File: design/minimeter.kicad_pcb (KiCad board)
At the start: 2 copper layers, 44.4 x 26.7 mm, 14 parts, among them J1 Conn_01x02_Pin, J2 I2C, SW1 SW_Push_Dual, SW2 SW_Push_Dual

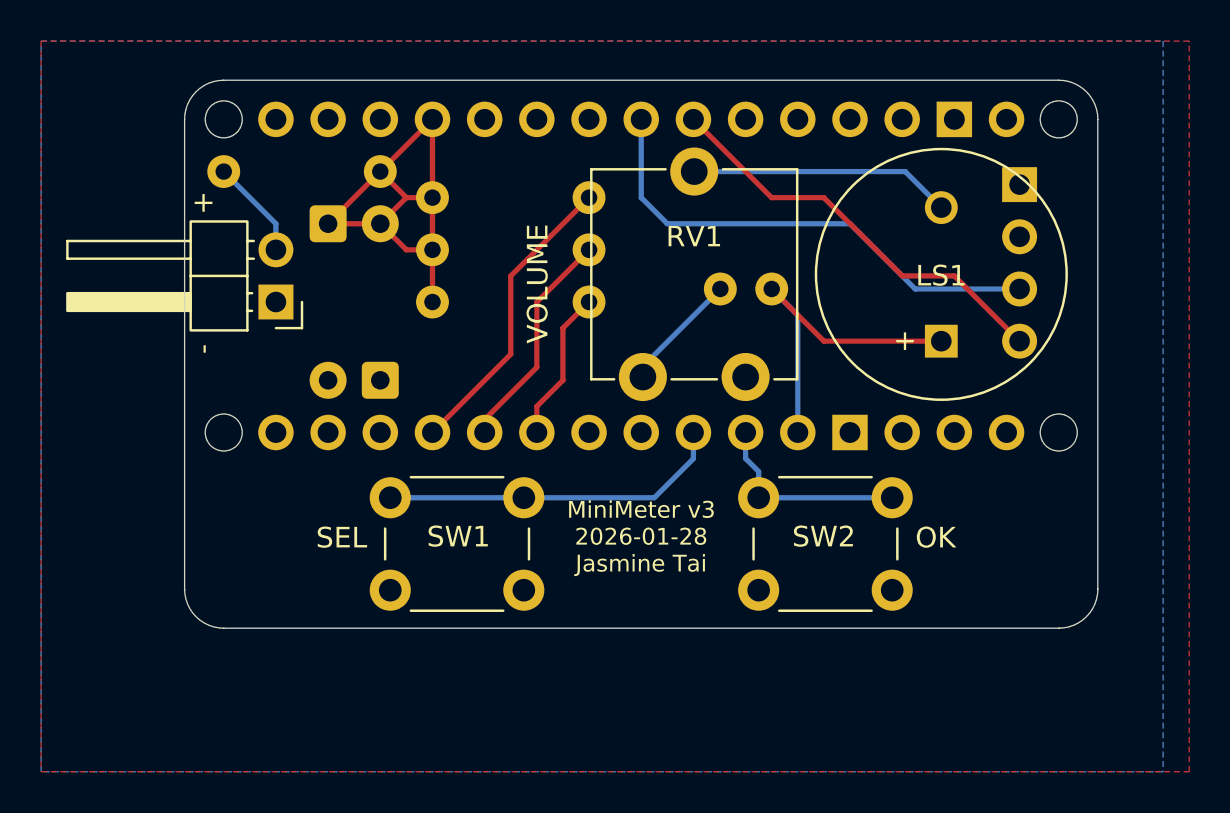
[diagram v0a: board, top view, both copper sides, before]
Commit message: Update design to v4
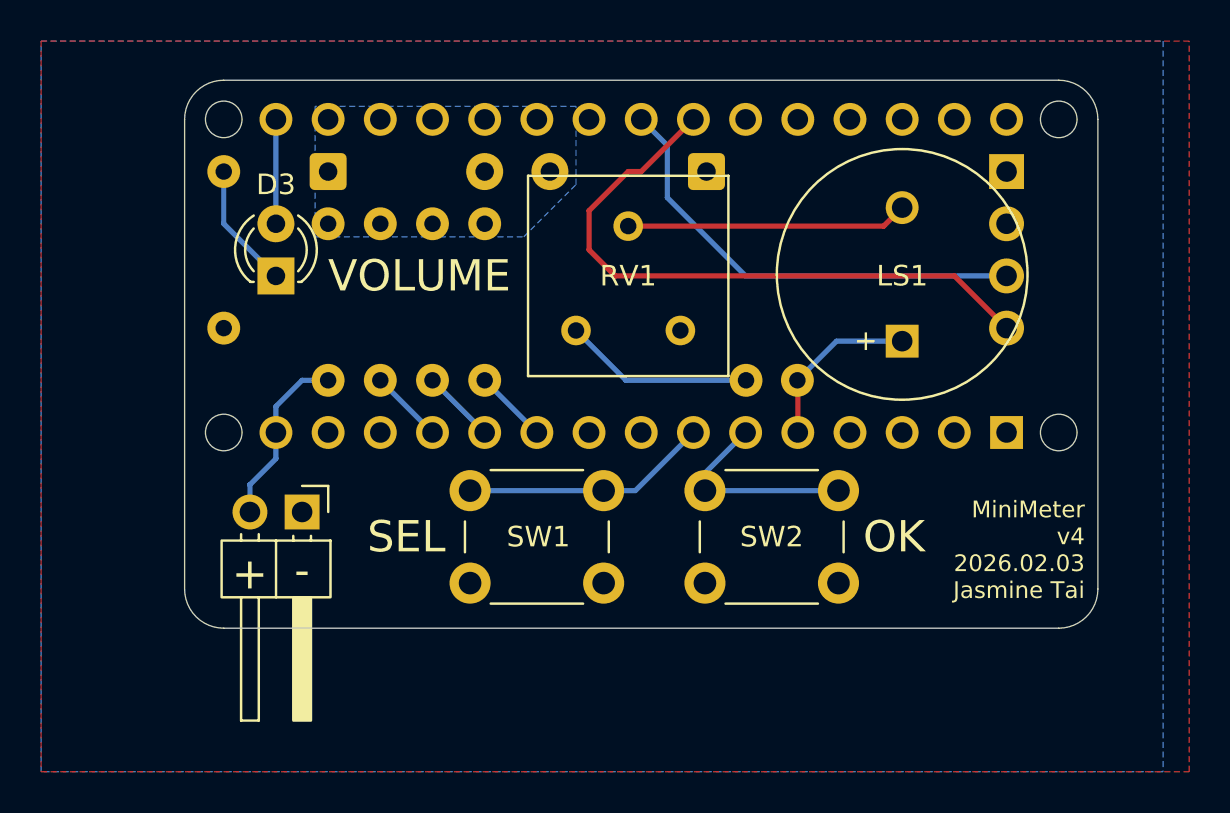
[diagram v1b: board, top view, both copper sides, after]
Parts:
- added D3: LED_Filled, LED_THT:LED_D3.0mm, F.Cu at (49.5, 57.1)
- added R5: 820, Resistor_THT:R_Axial_DIN0207_L6.3mm_D2.5mm_P7.62mm_Horizontal, B.Cu at (47.0, 59.7)
- A1: footprint arduino-library:Arduino_Nano_Socket -> Module:Arduino_Nano_WithMountingHoles
- RV1: footprint Potentiometer_THT:Potentiometer_ACP_CA9-V10_Vertical -> Potentiometer_THT:Potentiometer_Bourns_3386F_Vertical
- moved A1 40.1 mm to (85.1, 64.8)
- moved D1 18.8 mm to (70.5, 52.1), turned to 180 degrees
- moved R1 11.4 mm to (52.1, 62.2), turned to 90 degrees
- moved J1 10.3 mm to (50.8, 68.6), turned to -90 degrees
- moved C1 4.62 mm to (74.9, 62.2)
- moved R4 4.58 mm to (59.7, 54.6), turned to -90 degrees
- moved SW1 3.90 mm to (59.0, 67.6)
- moved RV1 3.90 mm to (69.2, 59.8)
- moved R2 2.84 mm to (54.6, 54.6), turned to -90 degrees
- moved SW2 2.64 mm to (70.4, 67.6)
- moved D2 2.54 mm to (52.1, 52.1), turned to 0 degrees
- moved LS1 1.91 mm to (80.0, 60.3)
- moved R3 1.27 mm to (57.1, 54.6), turned to -90 degrees
- moved J2 0.90 mm to (85.1, 52.1)
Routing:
- net /IN_PROT: track 26.5 -> 0.00 mm
- net /PULL_4.7K: track 14.6 -> 3.59 mm
- net /SCL: track 20.3 -> 30.7 mm
- net /SPKR: track 16.8 -> 8.44 mm
- net /PULL_1K: track 11.0 -> 3.59 mm
- net Net-(D3-K): track 0.00 -> 6.13 mm
- net /LED: track 0.00 -> 5.08 mm
- net /BTN_SEL: track 16.8 -> 12.0 mm
- net /IN: track 4.86 -> 8.73 mm
- net /PULL_100: track 7.40 -> 3.59 mm
- net Net-(C1-Pad2): track 6.01 -> 9.28 mm
- net /SDA: track 24.1 -> 22.4 mm
- net Net-(LS1--): track 12.8 -> 13.7 mm
- added copper zone on B.Cu, net /IN_PROT
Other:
- board text added: "MiniMeter v4 2026.02.03 Jasmine Tai"
- board text removed: "MiniMeter v3 2026-01-28 Jasmine Tai"
- board text removed: "USB SIDE"
